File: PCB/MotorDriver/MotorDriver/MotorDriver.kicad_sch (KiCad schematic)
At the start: 75 parts, among them J13 JST-XH, J14 JST-XH, J2 JST-XH, J3 XT30PW-M, J5 JST-XH, J6 JST-XH, J7 JST-XH, J8 JST-XH, J9 JST-XH, Q10 NMOS, Q3 TJ60S04M3L, SW1 SW_Push, SW2 SW_DPST_x2, U1 Pico, U15 AZ1117CH-3.3TR, U3 TCA9548APWR

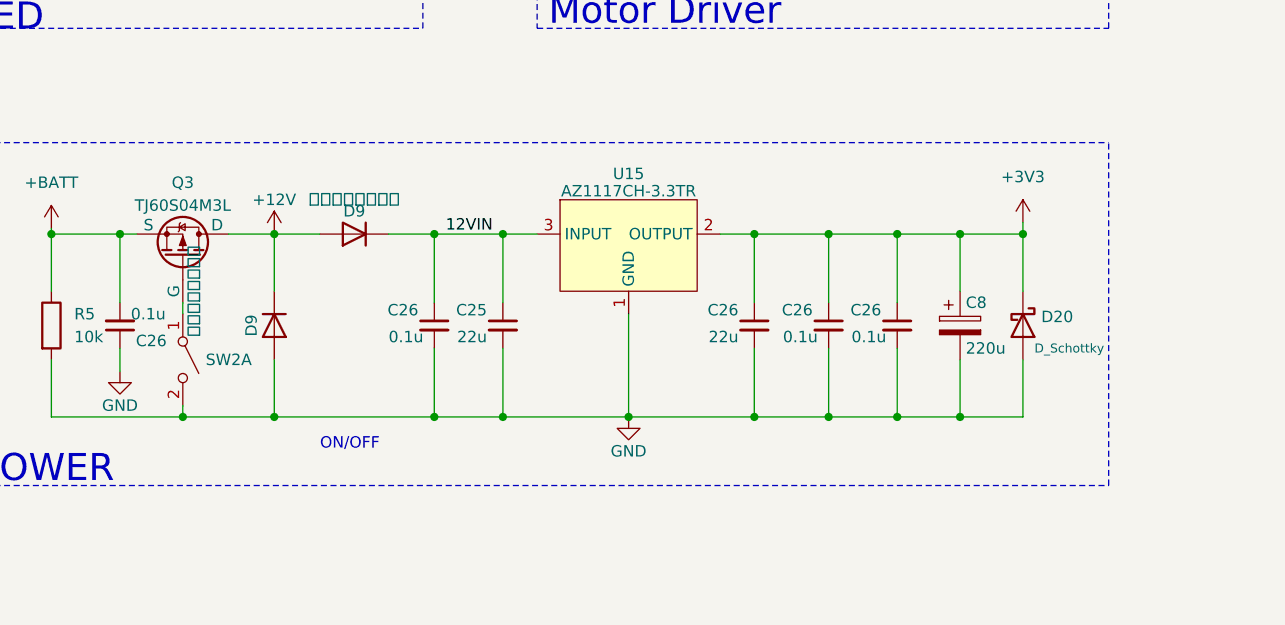
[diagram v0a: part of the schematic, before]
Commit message: ✏️ 昔のファイルを引っ張てきた
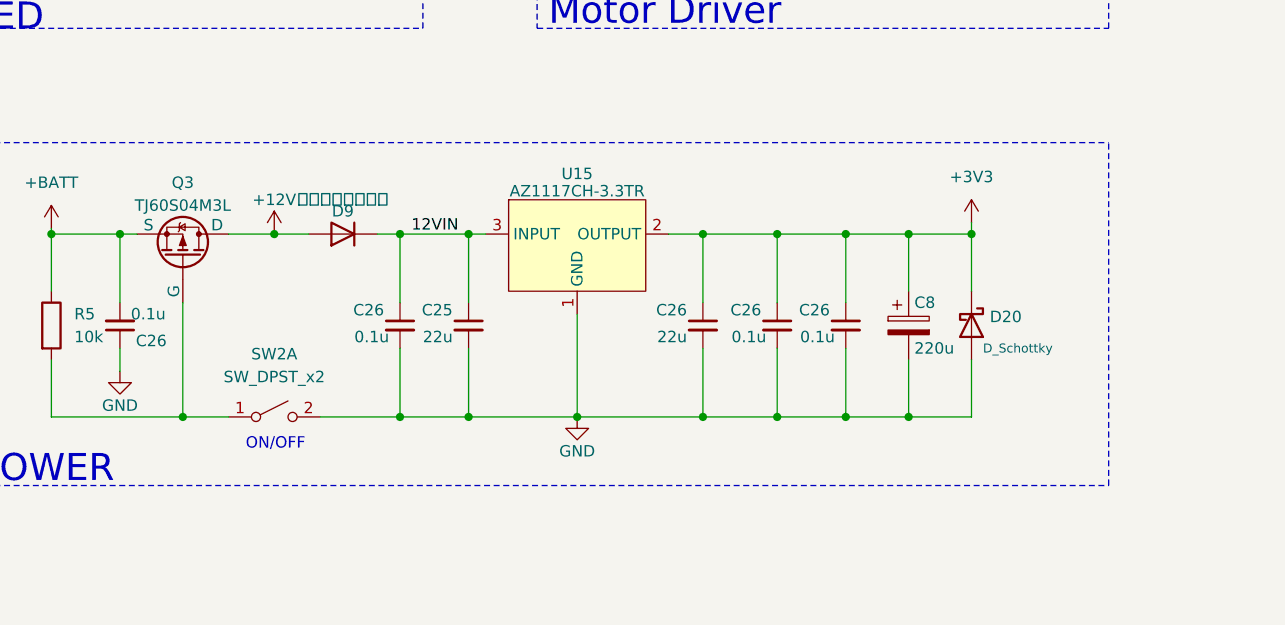
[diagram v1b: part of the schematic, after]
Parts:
- removed D9: ＧＳ１０１０ＦＬ, Diode_SMD:D_SOD-123F, symbol Device:D
- Q10: footprint TPH11006NL:TPH11006NL_SOP Advance_TOS-M -> Package_TO_SOT_SMD:SOT-23
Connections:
- net GND: no longer R5.2
- net at Q3.1 (G), SW2.1 (A): now also R5.2
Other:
- moved on the sheet: C25, C26, C8, D20, D9, SW2A, U15

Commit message: :sparkles: Production Done
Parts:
- Q10: footprint Package_TO_SOT_SMD:SOT-23 -> TPH11006NL:TPH11006NL_SOP Advance_TOS-M
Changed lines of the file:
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@@
       (effects (font (size 1.27 1.27)) (justify left))
     )
-    (property "Footprint" "Package_TO_SOT_SMD:SOT-23" (at 154.94 86.36 0)
+    (property "Footprint" "TPH11006NL:TPH11006NL_SOP Advance_TOS-M" (at 154.94 86.36 0)
       (effects (font (size 1.27 1.27)) hide)
     )
